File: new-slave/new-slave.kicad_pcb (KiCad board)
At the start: 2 copper layers, 26.2 x 71.6 mm, 9 parts, among them J1 Conn_01x06_Male, J2 Conn_01x06_Male, J3 Conn_01x06_Female, J4 Screw_Terminal_01x03, U1 RS485-TTL-Board

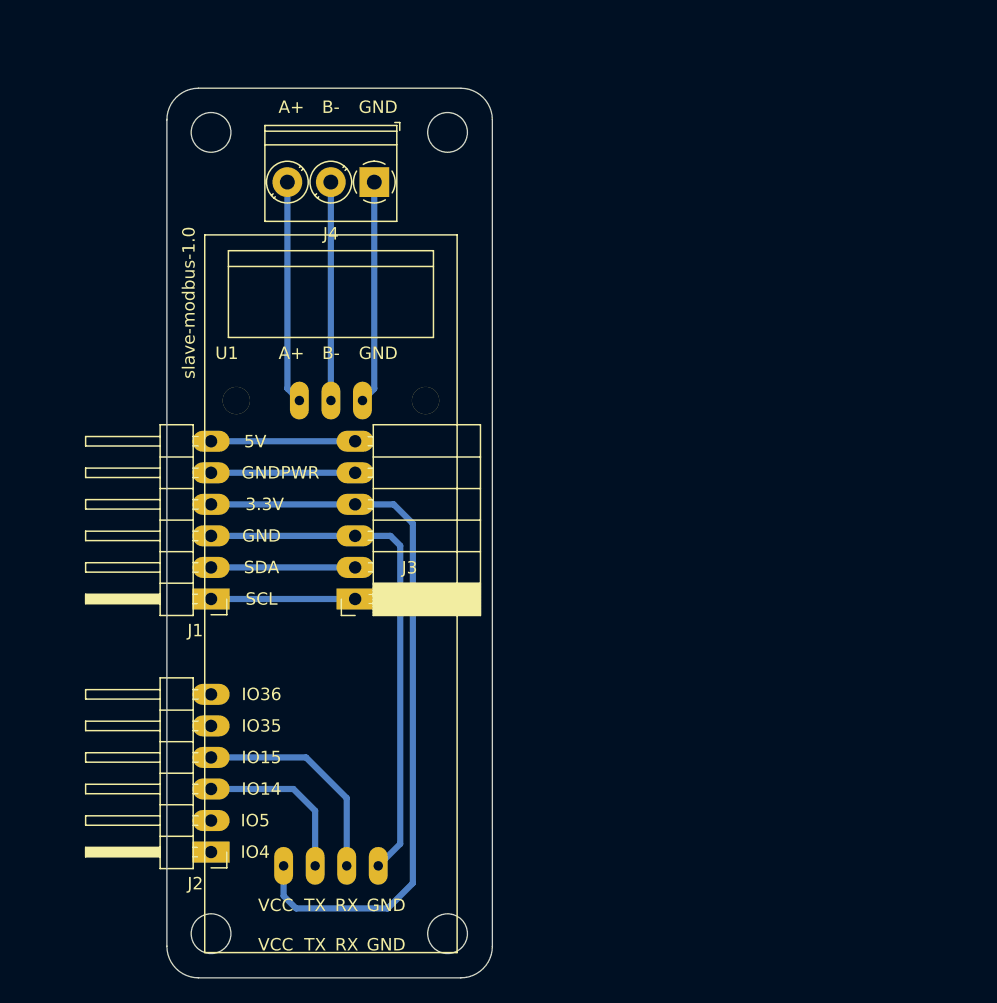
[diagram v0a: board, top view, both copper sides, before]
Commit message: slave-modbus-1.0
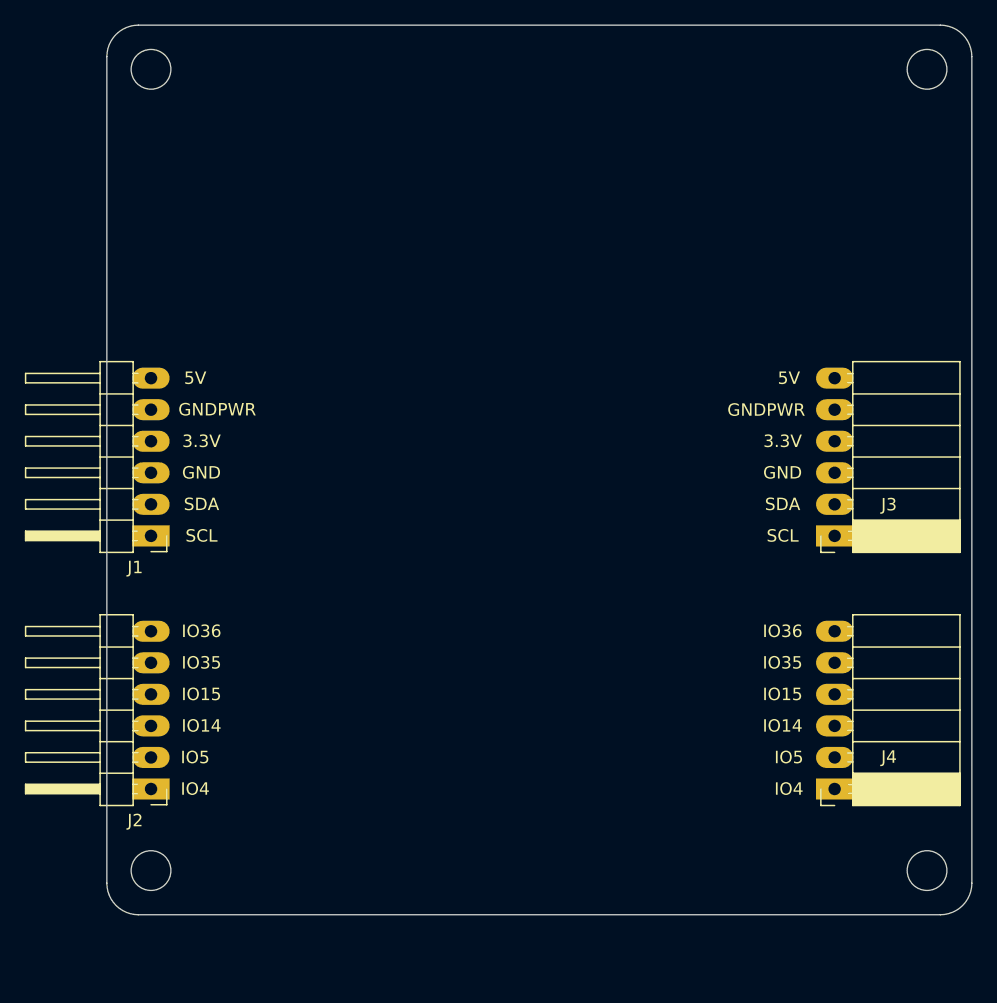
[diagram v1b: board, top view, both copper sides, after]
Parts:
- removed U1: RS485-TTL-Board, boards:RS485-TTL-Board-DsdTech
- J4: value Screw_Terminal_01x03 -> Conn_01x06_Female; footprint TerminalBlock_Phoenix:TerminalBlock_Phoenix_PT-1,5-3-3.5-H_1x03_P3.50mm_Horizontal -> Connector_PinSocket_2.54mm:PinSocket_1x06_P2.54mm_Horizontal
- moved J4 61.3 mm to (122.1, 116.9)
- moved H2 38.9 mm to (129.5, 58.9)
- moved H4 38.9 mm to (129.5, 123.4)
- moved J3 38.9 mm to (122.1, 96.5)
- moved H1 7.01 mm to (67.1, 58.9)
- moved H3 7.01 mm to (67.1, 123.4)
- moved J1 7.01 mm to (67.1, 96.5)
- moved J2 7.01 mm to (67.1, 116.9)
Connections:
- net +24V renamed +5V
- J4 pad 1: Net-(J4-Pad1) -> GPIO4
- J4 pad 2: Net-(J4-Pad2) -> GPIO5
- J4 pad 3: Net-(J4-Pad3) -> GPIO14
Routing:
- net +3V3: track 59.9 -> 0.00 mm
- net GND: track 42.1 -> 0.00 mm
- net Net-(J4-Pad3): track 18.0 -> 0.00 mm
- net Net-(J4-Pad1): track 18.0 -> 0.00 mm
- net GPIO15: track 17.7 -> 0.00 mm
- net Net-(J4-Pad2): track 17.6 -> 0.00 mm
- net GPIO14: track 13.5 -> 0.00 mm
- net SDA: track 11.6 -> 0.00 mm
- net SCL: track 11.6 -> 0.00 mm
- net GNDPWR: track 11.6 -> 0.00 mm
- net +5V: track 11.6 -> 0.00 mm
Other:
- board size 26.2 x 71.6 mm -> 69.6 x 71.6 mm
- board text removed: "A+"
- board text removed: "B-"
- board text removed: "slave-modbus-1.0"
